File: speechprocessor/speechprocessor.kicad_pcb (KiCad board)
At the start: 2 copper layers, 10.8 x 7 mm, 6 parts

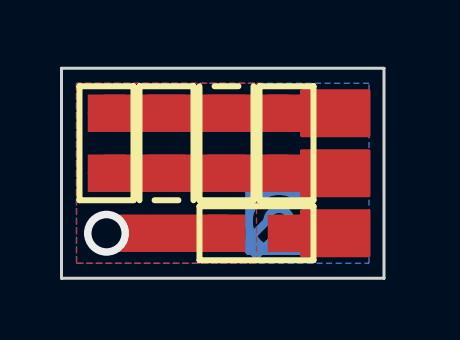
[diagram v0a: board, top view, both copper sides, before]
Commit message: Update for manufacture
Signed-off-by: Andres Gongora <mail@andresgongora.com>
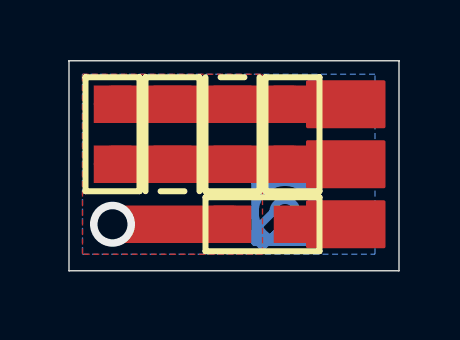
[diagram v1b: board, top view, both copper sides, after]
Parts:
- moved D1 0.36 mm to (127.5, 111.5)
- moved D2 0.36 mm to (125.5, 111.5)
- moved e 0.36 mm to (123.5, 111.5)
- moved C1 0.36 mm to (129.4, 111.5)
- moved C2 0.36 mm to (128.4, 114.5)
- moved Ref** 0.36 mm to (129.2, 114.5)
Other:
- board size 10.8 x 7 mm -> 11 x 7 mm
